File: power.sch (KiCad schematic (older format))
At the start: 46 parts, among them IC1 TPS65217C, U1 AP2112K-3.3TRG1, U2 AP2112K-1.8TRG1, U3 TL1963A-33DCQR

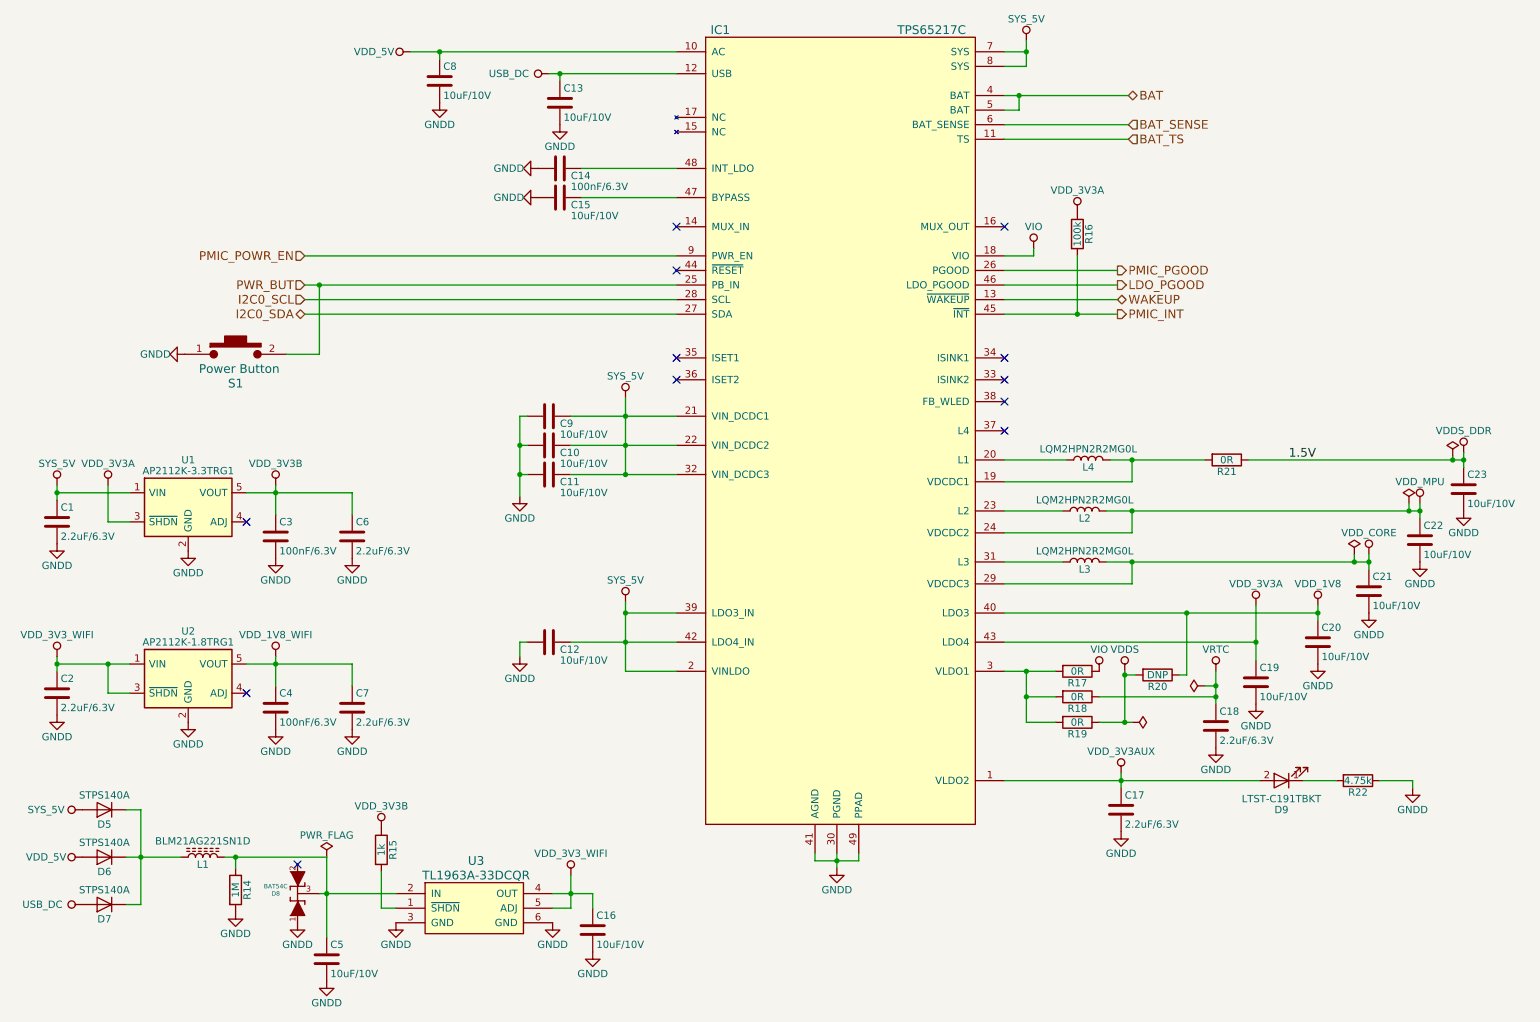
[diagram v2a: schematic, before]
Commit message: wip sys and power
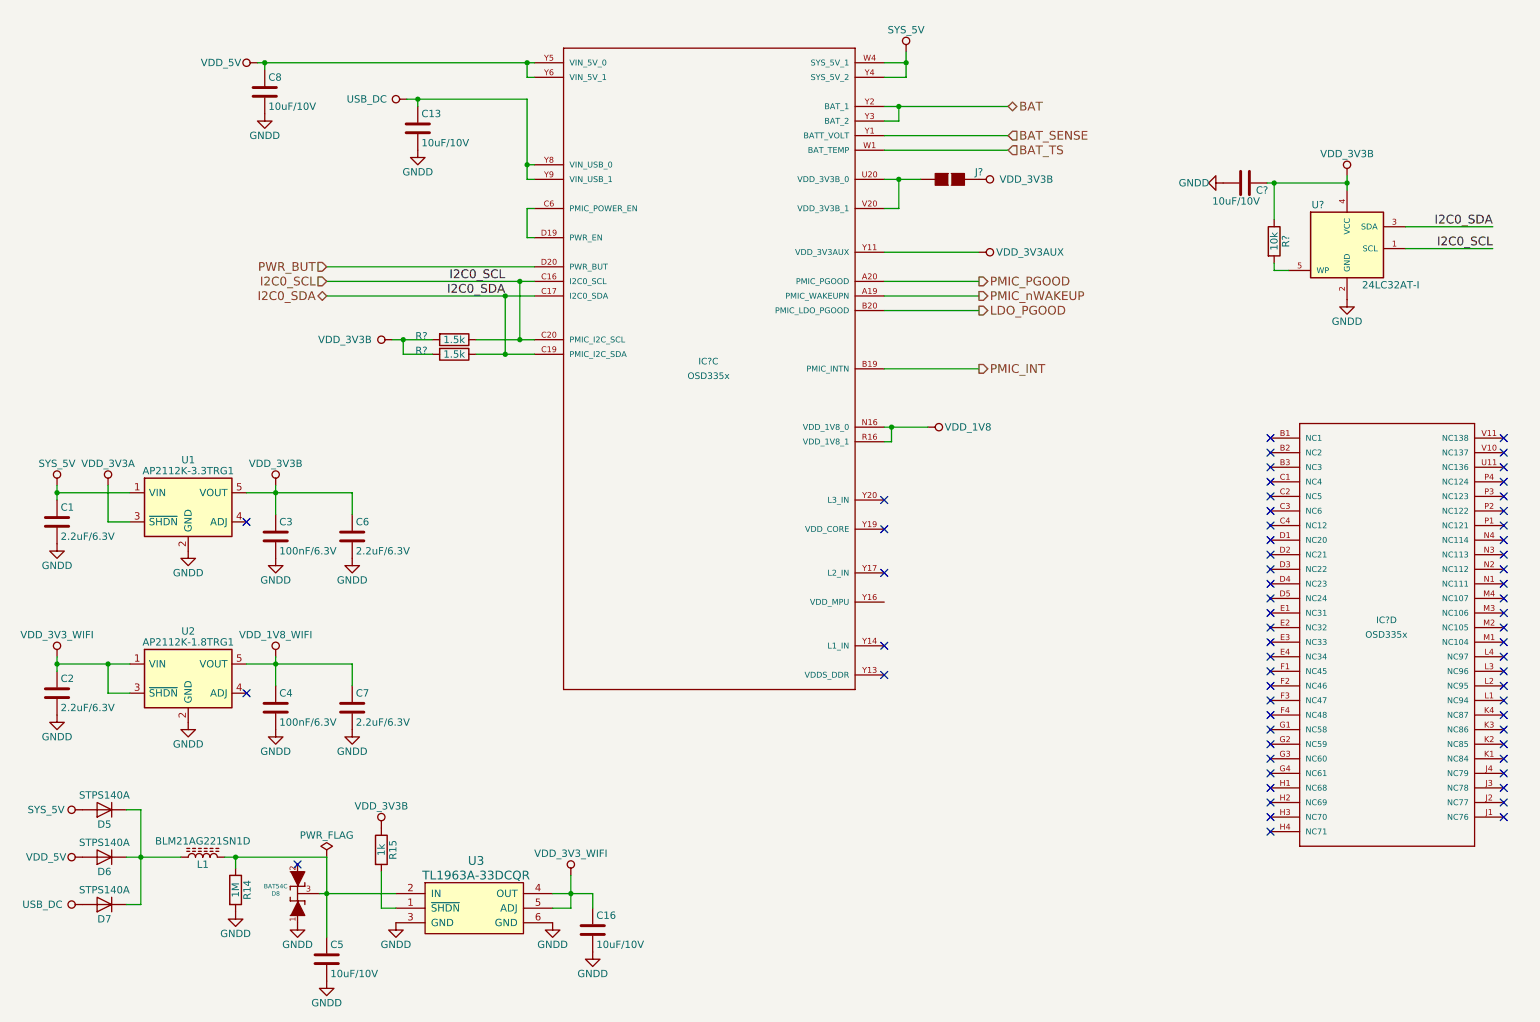
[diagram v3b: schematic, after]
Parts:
- removed C10, C11, C12, C15, C19, C20, C21, C22, C23, C9: 10uF/10V, symbol C
- removed C14: 100nF/6.3V, symbol C
- removed C17, C18: 2.2uF/6.3V, symbol C
- removed D9: LTST-C191TBKT, symbol LED
- removed IC1: TPS65217C, symbol TPS65217C
- removed L2, L3, L4: LQM2HPN2R2MG0L, symbol L
- removed R16: 100k, symbol R
- removed R17, R18, R19, R21: 0R, symbol R
- removed R20: DNP, symbol R
- removed R22: 4.75k, symbol R
- removed S1: Power Button, symbol PushButton
- added C?: 10uF/10V, symbol C
- added IC? (x2): OSD335x, GHI-SoMs-Processors_OSD3358, symbol OSD335x
- added J?: GS2, Connectors:GS2, symbol GS2
- added R? (x2): 1.5k, symbol R
- added R?: 10k, symbol R
- added U?: 24LC32AT-I, TO_SOT_Packages_SMD:SOT-23-5, symbol AT24CS32-STUM
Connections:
- net BAT: now also IC?.Y2 (BAT_1), IC?.Y3 (BAT_2)
- net BAT_SENSE: now also IC?.Y1 (BATT_VOLT)
- net BAT_TS: now also IC?.W1 (BAT_TEMP)
- net GNDD: now also C?.2, U?.2 (GND)
- net I2C0_SCL: now also IC?.C16 (I2C0_SCL), IC?.C20 (PMIC_I2C_SCL), R?.1, U?.1 (SCL)
- net I2C0_SDA: now also IC?.C17 (I2C0_SDA), IC?.C19 (PMIC_I2C_SDA), R?.1, U?.3 (SDA)
- net LDO_PGOOD: now also IC?.B20 (PMIC_LDO_PGOOD)
- net PMIC_INT: now also IC?.B19 (PMIC_INTN)
- net PMIC_PGOOD: now also IC?.A20 (PMIC_PGOOD)
- net PWR_BUT: now also IC?.D20 (PWR_BUT)
- net SYS_5V: now also IC?.W4 (SYS_5V_1), IC?.Y4 (SYS_5V_2)
- net USB_DC: now also IC?.Y8 (VIN_USB_0), IC?.Y9 (VIN_USB_1)
- net VDD_1V8: now also IC?.N16 (VDD_1V8_0), IC?.R16 (VDD_1V8_1)
- net VDD_3V3AUX: now also IC?.Y11 (VDD_3V3AUX)
- net VDD_3V3B: now also C?.1, J?.1 (G1), R?.1, R?.2, R?.2, U?.4 (VCC)
- net VDD_5V: now also IC?.Y5 (VIN_5V_0), IC?.Y6 (VIN_5V_1)
- new net: IC?.C6 (PMIC_POWER_EN), IC?.D19 (PWR_EN)
- new net: IC?.U20 (VDD_3V3B_0), IC?.V20 (VDD_3V3B_1), J?.2 (G2)
- new net: R?.2, U?.5 (WP)
- new net PMIC_nWAKEUP: IC?.A19 (PMIC_WAKEUPN)
- no-connect marks 12 -> 63
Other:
- moved on the sheet: C13, C8
